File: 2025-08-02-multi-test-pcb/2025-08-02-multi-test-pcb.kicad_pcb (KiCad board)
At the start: 2 copper layers, 102.9 x 53.3 mm, 6 parts, among them J1 Conn_02x15_Odd_Even

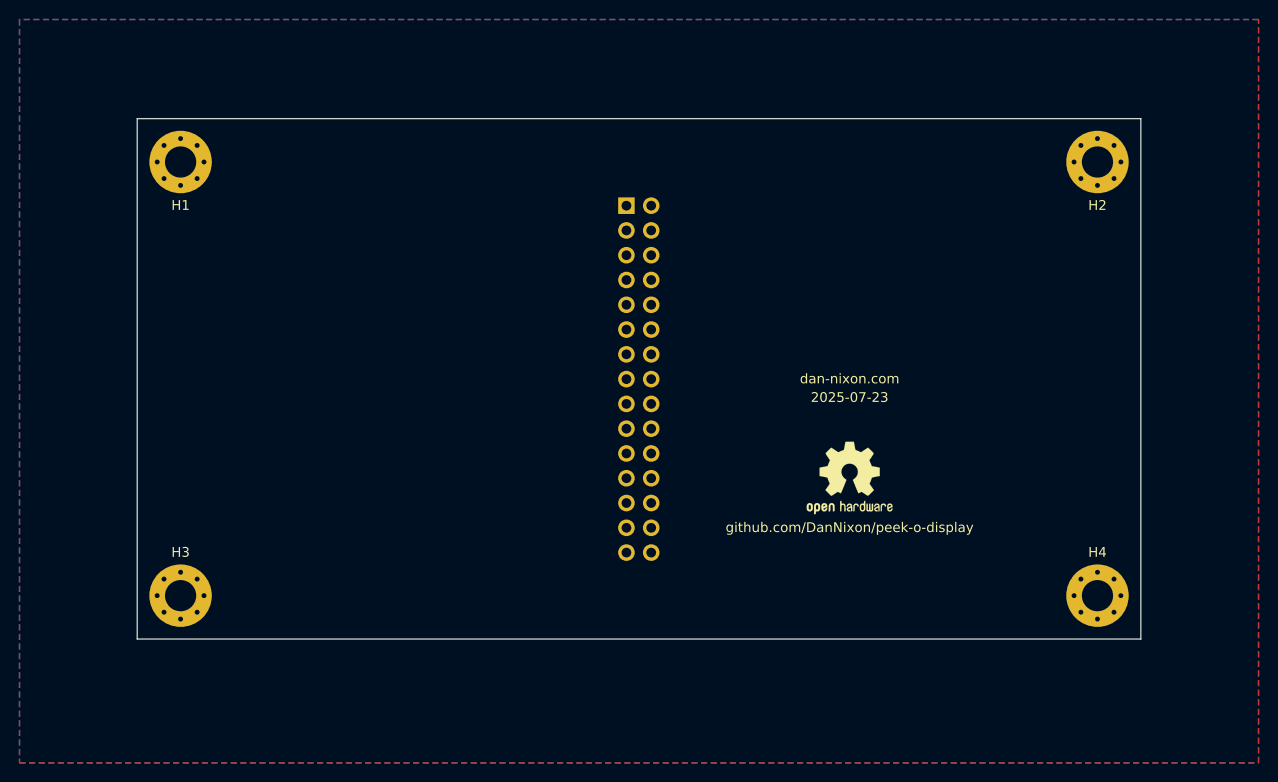
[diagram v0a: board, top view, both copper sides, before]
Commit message: wip
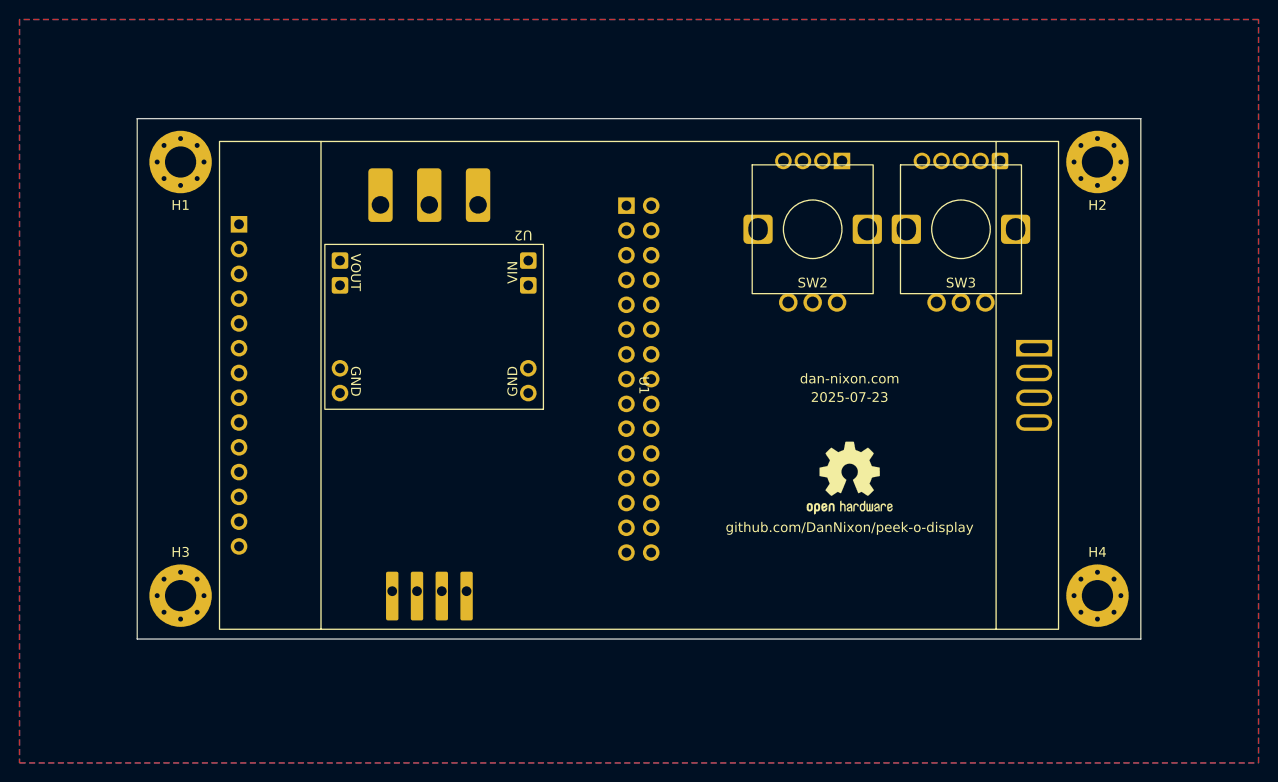
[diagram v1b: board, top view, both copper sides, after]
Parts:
- added SW2: RotaryEncoder_Switch_RG, Input:RotaryEncoder_Switch_RG, F.Cu at (144.8, 85.0)
- added SW3: RotaryEncoder_Switch_RGB, Input:RotaryEncoder_Switch_RGB, F.Cu at (160.0, 85.0)
- added U1: ~, Displays:ILI9341_2.8in_with_touch_and_sd, F.Cu at (127.0, 101.0)
- added U2: ~, Modules:AliE_MP1584EN_regulator, F.Cu at (106.0, 95.0)
- added U3: RS485 to TTL module, Modules:RS485_to_ttl, B.Cu at (105.5, 102.0)
